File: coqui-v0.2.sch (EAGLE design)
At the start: 20 parts, among them IC3 MCP73831, IC4 MCP1700-33, J1 AYZ0202, X1 USBSMD

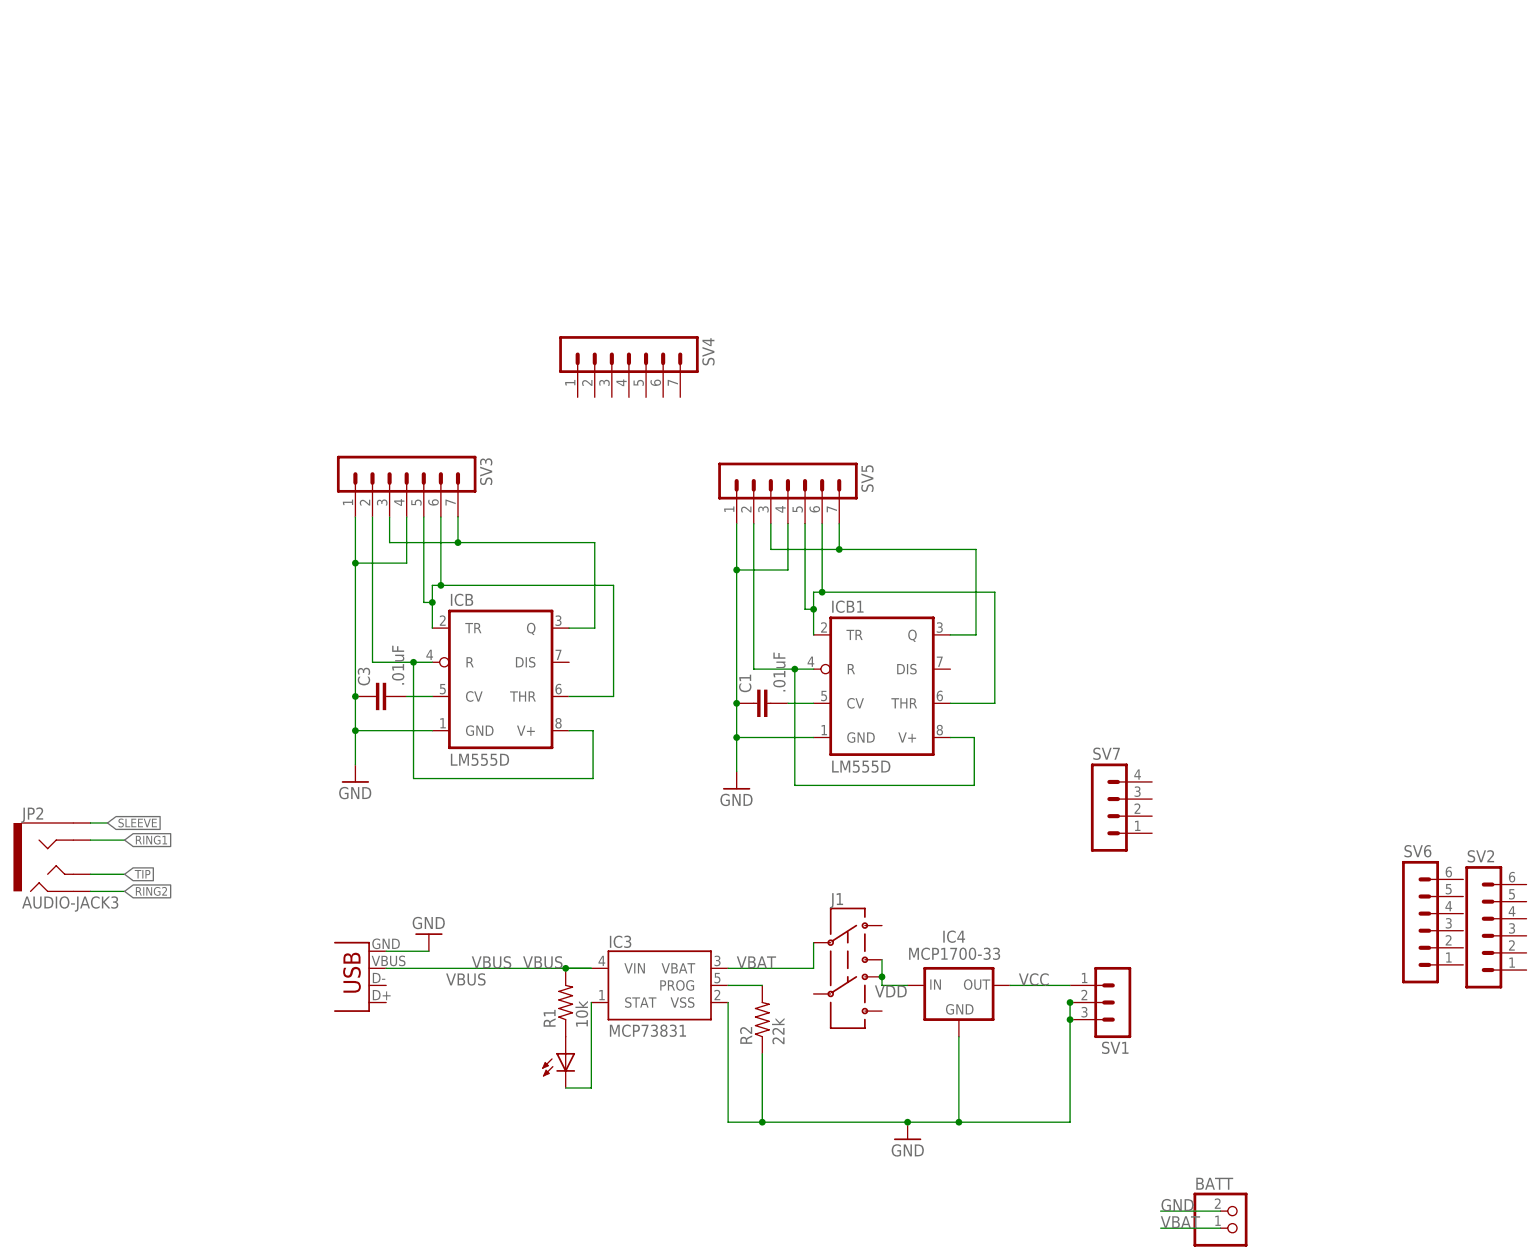
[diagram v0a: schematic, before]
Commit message: update
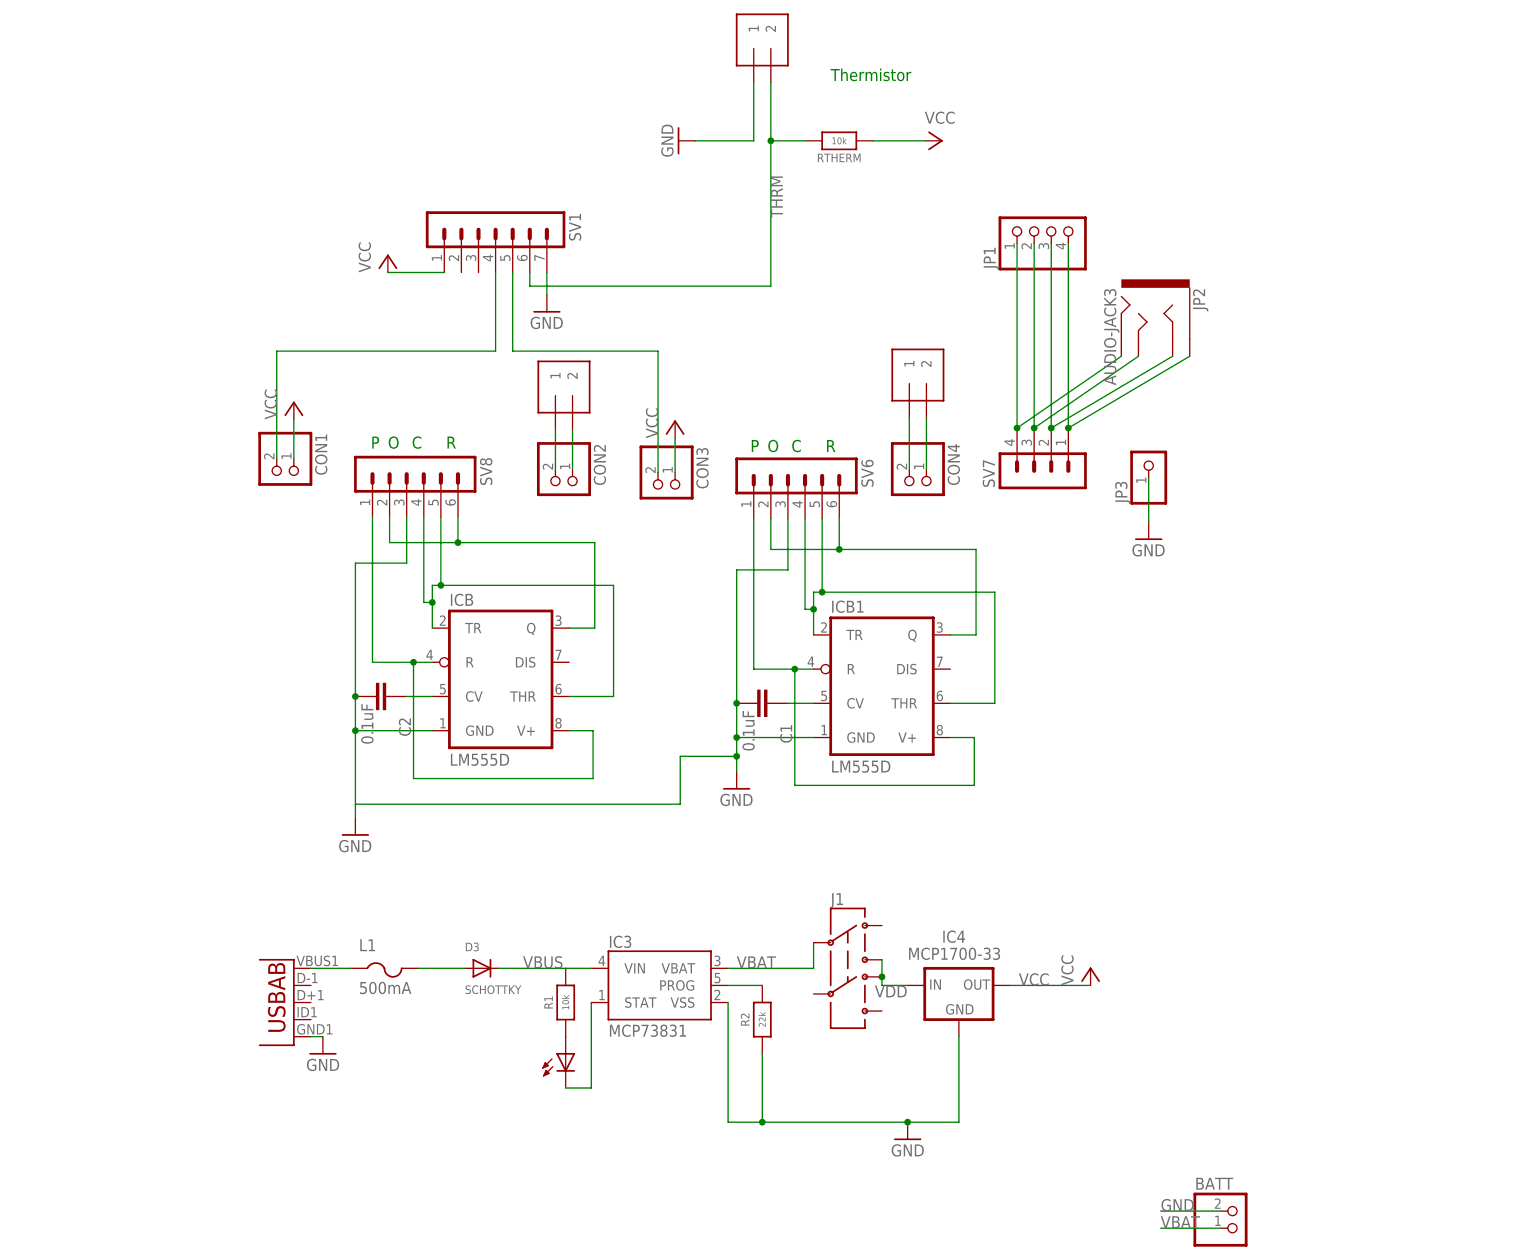
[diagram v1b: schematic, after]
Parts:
- removed C3: .01uF, SparkFun:CAP0402-CAP
- removed SV2: (no value), con-lstb:MA06-1
- removed SV3, SV4, SV5: (no value), con-lstb:MA07-1
- removed X1: USBSMD, SparkFun:USBSMD
- added C2: 0.1uF, SparkFun:CAP0603-CAP
- added CON1, CON2, CON3, CON4: (no value), pinhead:PINHD-1X2
- added D3: SCHOTTKY, adafruit:DIODE_SOD-123FL
- added IN1, IN2, THRM: 1X2-3.5MM, adafruit:1X2-3.5MM
- added JP1: (no value), trrs-dwb:PINHD-1X4/90
- added JP3: (no value), pinhead:PINHD-1X1
- added L1: 500mA, adafruit:PTCFUSE-1206
- added RTHERM: 10k, microbuilder:RESISTOR_0603_NOOUT
- added SV8: (no value), con-lstb:MA06-1
- added U$4: (no value), Testing:USB-AB""
- C1: value .01uF -> 0.1uF; device SparkFun:CAP0402-CAP -> SparkFun:CAP0603-CAP
- R1, R2: device SparkFun:RESISTOR0402-RES -> microbuilder:RESISTOR_0603_NOOUT
- SV1: device con-lstb:MA03-1 -> con-lstb:MA07-1
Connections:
- removed net RING1: JP2.RING1
- removed net RING2: JP2.RING2
- removed net SLEEVE: JP2.EARTH
- removed net TIP: JP2.TIP
- new net N$10: CON2.2, IN1.1
- new net N$12: L1.1, U$4.VBUS
- new net N$13: D3.A, L1.2
- new net N$15: CON2.1, IN1.2
- new net N$16: CON4.2, IN2.1
- new net N$17: CON4.1, IN2.2
- new net N$18: CON1.2, SV1.4
- new net N$19: CON3.2, SV1.5
- new net N$6: JP1.4, JP2.EARTH, SV7.1
- new net N$7: JP1.3, JP2.RING1, SV7.2
- new net N$8: JP1.2, JP2.TIP, SV7.3
- new net N$9: JP1.1, JP2.RING2, SV7.4
- new net THRM: RTHERM.2, SV1.6, THRM.2
- net AOUT: now also SV8.2, SV8.6; no longer SV3.3, SV3.7
- net AOUT1: now also SV6.2, SV6.6; no longer SV5.3, SV5.7
- net GND: now also C2.1, JP3.1, SV1.7, SV6.3, SV8.3, THRM.1, U$4.GND; no longer C3.1, SV1.2, SV1.3, SV3.1, SV3.4, SV5.1, SV5.4, X1.GND
- net N$1: now also SV6.4, SV6.5; no longer SV5.5, SV5.6
- net N$11: now also SV8.4, SV8.5; no longer SV3.5, SV3.6
- net N$14: now also C2.2; no longer C3.2
- net VAIN: now also SV8.1; no longer SV3.2
- net VAIN1: now also SV6.1; no longer SV5.2
- net VBUS: now also D3.C; no longer IC3.VIN, X1.VBUS
- net VCC: now also CON1.1, CON3.1, RTHERM.1
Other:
- note added: "C"
- note added: "O"
- note added: "P"
- note added: "R"
- note added: "Thermistor"
- moved on the sheet: JP2, SV6, SV7
